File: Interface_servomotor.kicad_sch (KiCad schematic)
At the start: 0 parts

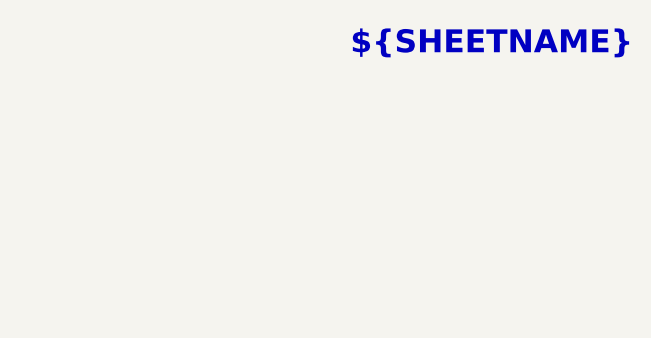
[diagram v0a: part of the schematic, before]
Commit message: testing green mask
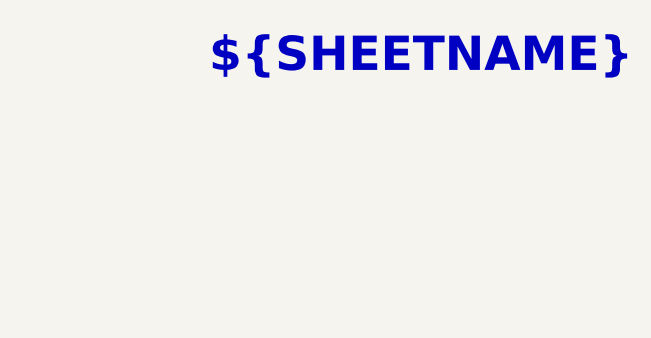
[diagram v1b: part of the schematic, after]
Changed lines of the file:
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@@
-		)
-	)
-	(text "${SHEETNAME}"
-		(exclude_from_sim no)
-		(at 283.21 13.97 0)
-		(effects
-			(font
-				(size 2.54 2.54)
-				(bold yes)
-			)
-			(justify right top)
 		)
 	)
@@
 		)
 	)
+	(text "${SHEETNAME}"
+		(exclude_from_sim no)
+		(at 283.21 14.605 0)
+		(effects
+			(font
+				(face "DejaVu Sans")
+				(size 3.81 3.81)
+				(bold yes)
+				(color 0 0 0 1)
+			)
+			(justify right top)
+		)
+	)

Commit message: reorganised sch and pcb
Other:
- note added: "JST B6B-XH-A / JST XHP-6 connector Pin Description 1 Encoder B output (VCC) 2 Encoder A output (VCC) 3 GND 4 VCC (3.3 - 5V) 5 Motor B (3 A, 12-24 V) 6 Motor A (3 A, 12-24 V)"
- note removed: "JST B6B-XH-A / JST XHP-6 connector Pin Description 1 Encoder B output (VCC) 2 Encoder A output (VCC)r 3 GND 4 VCC (3.3 - 5V)r 5 Motor B (3 A, 12-24 V)r 6 Motor A (3 A, 12-24 V)"
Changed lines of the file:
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@@
 	(generator_version "10.0")
 	(paper "A4")
-	(text "JST B6B-XH-A / JST XHP-6 connector\n\nPin  Description\n  1  Encoder B output (VCC)\n  2  Encoder A output (VCC)\r\n  3  GND\n  4  VCC (3.3 - 5V)\r\n  5  Motor B (3 A, 12-24 V)\r\n  6  Motor A (3 A, 12-24 V)"
+	(text "JST B6B-XH-A / JST XHP-6 connector\n\nPin  Description\n  1  Encoder B output (VCC)\n  2  Encoder A output (VCC)\n  3  GND\n  4  VCC (3.3 - 5V)\n  5  Motor B (3 A, 12-24 V)\n  6  Motor A (3 A, 12-24 V)"
 		(exclude_from_sim no)
 		(at 26.035 31.75 0)
